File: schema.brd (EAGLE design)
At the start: 31.4 x 38.1 mm, 7 parts, among them X1 BU-SMA-G

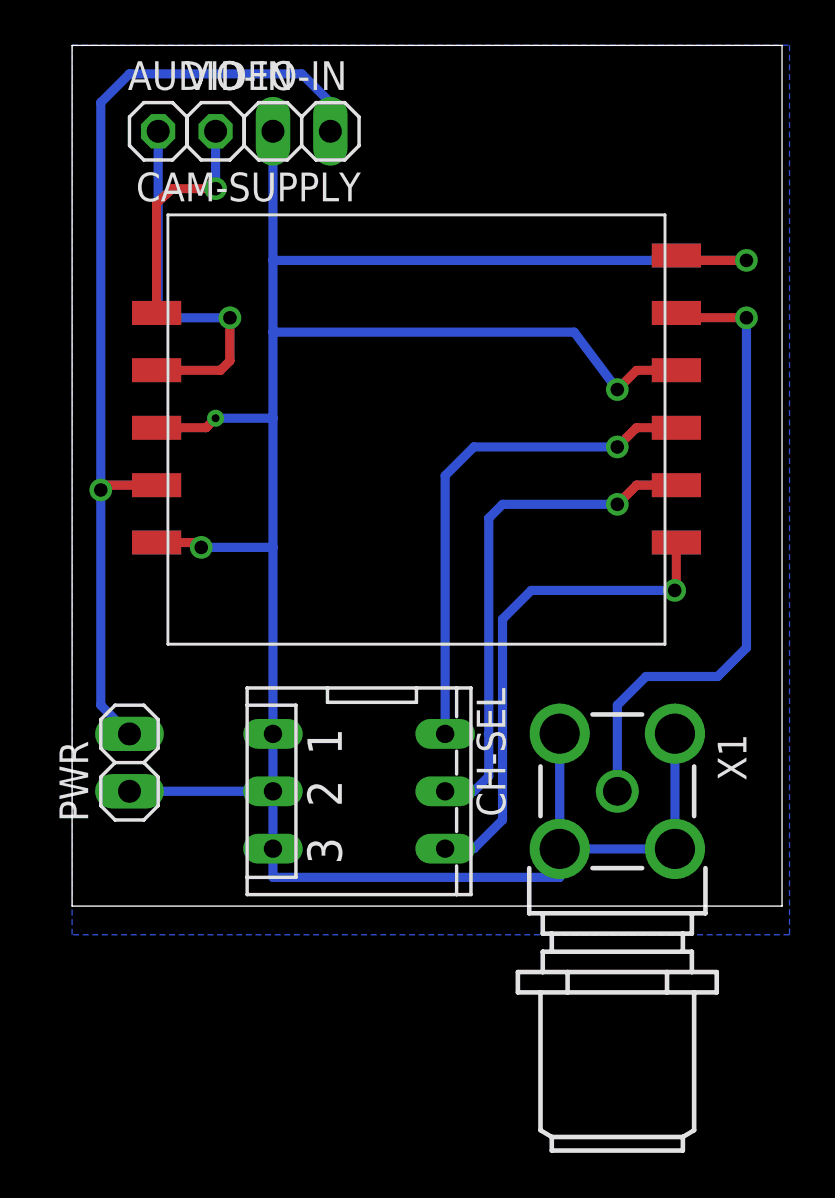
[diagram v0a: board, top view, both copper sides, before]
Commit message: Minor adjustments
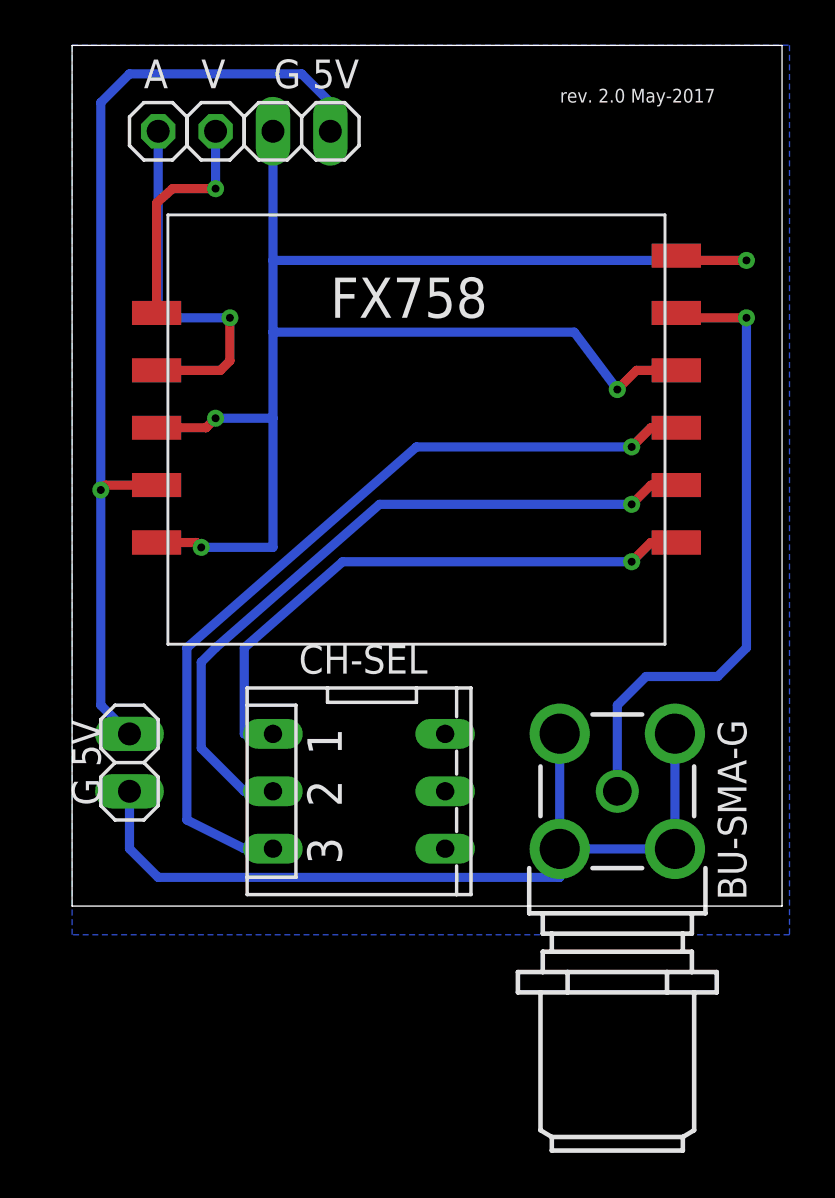
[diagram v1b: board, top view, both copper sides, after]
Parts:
- AUDIO-IN: value (none) -> A
- CAM-SUPPLY, PWR: value (none) -> G 5V
- VIDEO-IN: value (none) -> V
- renumbered X1 to SMA
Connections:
- net CH1: now also CH-SEL.1; no longer CH-SEL.4
- net CH2: now also CH-SEL.2; no longer CH-SEL.5
- net CH3: now also CH-SEL.3; no longer CH-SEL.6
- net GND: now also CH-SEL.4, CH-SEL.5, CH-SEL.6; no longer CH-SEL.1, CH-SEL.2, CH-SEL.3
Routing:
- net CH3: track 22.5 -> 37.1 mm
- net GND: track 122.8 -> 111.3 mm
- net CH2: track 22.6 -> 31.8 mm
- net CH1: track 22.3 -> 26.0 mm
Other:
- board text added: "FX758"
- board text added: "rev. 2.0 May-2017"
